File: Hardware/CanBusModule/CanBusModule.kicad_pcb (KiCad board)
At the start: 4 copper layers, 35.6 x 22.8 mm, 17 parts, among them U1 XIAO-ESP32-S3-Plus-SMD, U2 MCP2518FDT-E_QBB, U3 ATA6561-GBQW-N, U4 74HCT1G125GW, Y1 ECS-400-15-33B-CTN-TR

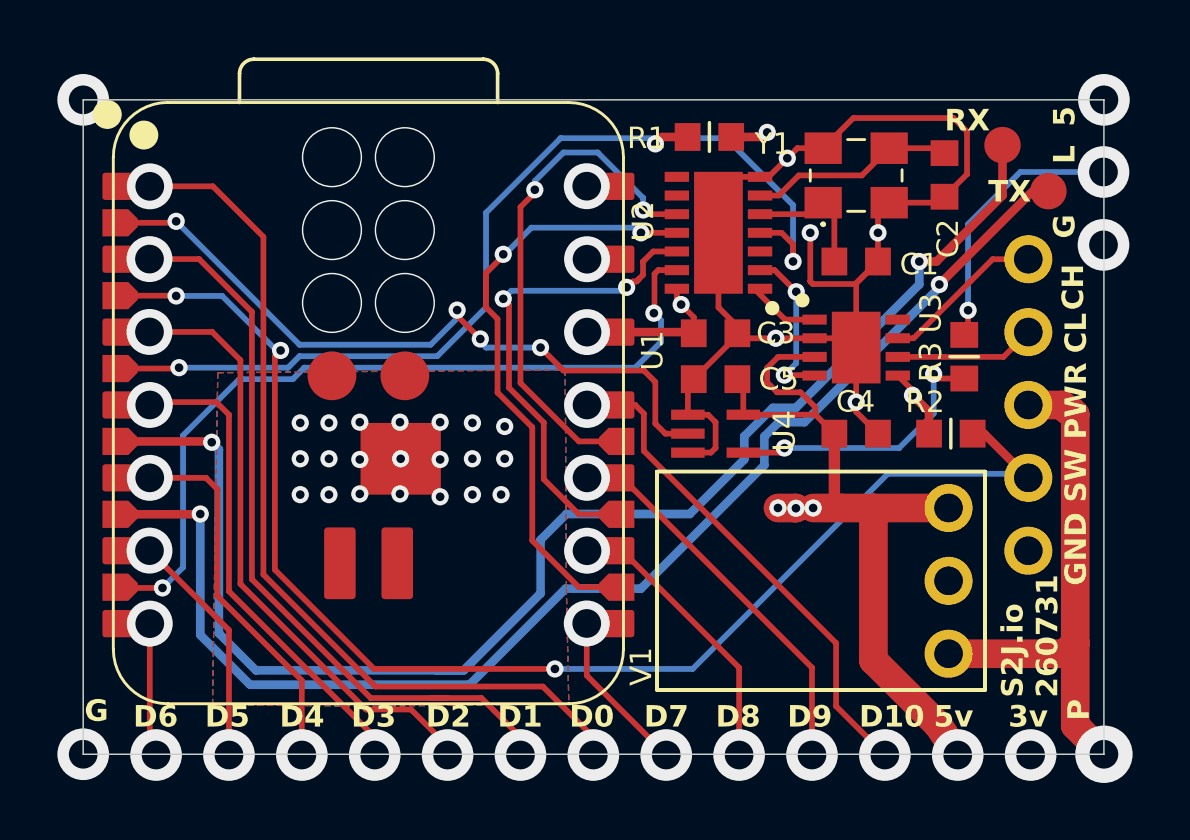
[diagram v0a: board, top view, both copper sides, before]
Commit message: Commiting an interim commit before chatgpt breaks it more
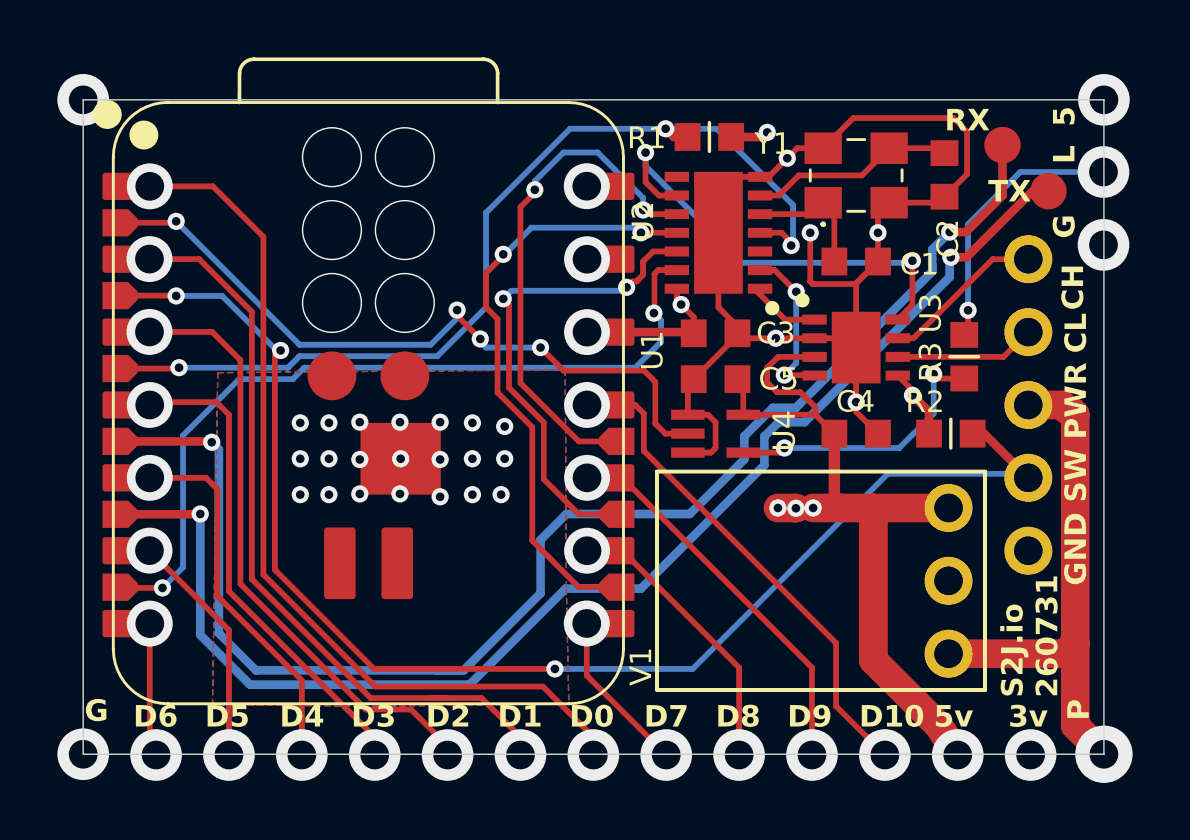
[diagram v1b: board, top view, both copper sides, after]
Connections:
- U2 pad 9: unconnected-(U2-~{INT0}/GPIO0/XSTBY-Pad9) -> Net-(U2-~{INT0}/GPIO0/XSTBY)
- U3 pad 8: unconnected-(U3-STBY-Pad8) -> Net-(U2-~{INT0}/GPIO0/XSTBY)
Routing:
- net Net-(U2-~{INT0}/GPIO0/XSTBY): track 0.00 -> 15.8 mm, vias 0 -> 2
- net /~{CANINT}: track 35.0 -> 33.8 mm
